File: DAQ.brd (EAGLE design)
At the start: 85.9 x 42.9 mm, 28 parts, among them IC1 PIC18F4550_40, IC2 7805T, Q1 20MHz, X1 PN61729-S

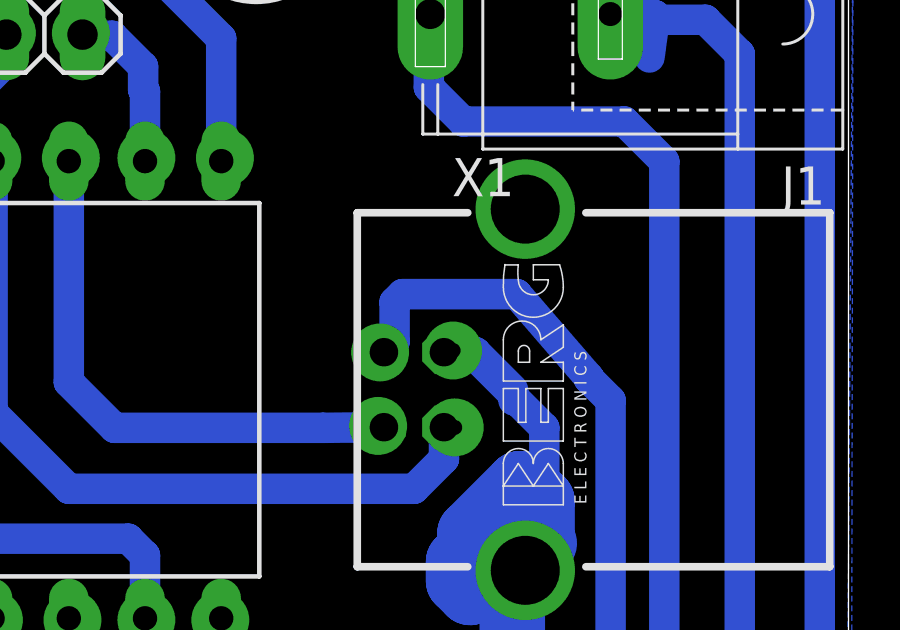
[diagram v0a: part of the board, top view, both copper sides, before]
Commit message: files word
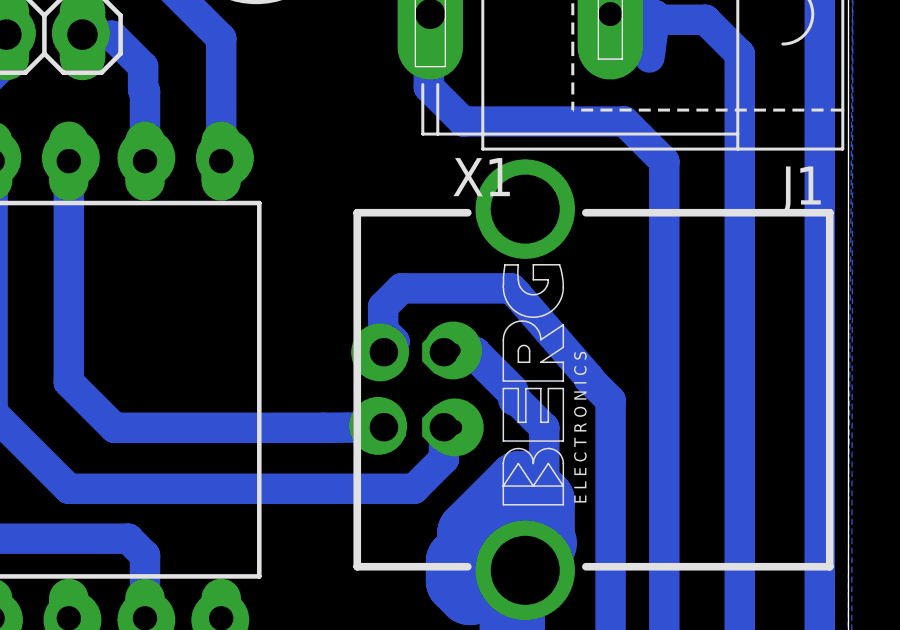
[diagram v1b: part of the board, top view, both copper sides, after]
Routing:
- net +5USB: track 175.3 -> 175.9 mm
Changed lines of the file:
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@@
 <layer number="14" name="Route14" color="1" fill="6" visible="no" active="no"/>
 <layer number="15" name="Route15" color="4" fill="6" visible="no" active="yes"/>
-<layer number="16" name="Bottom" color="1" fill="1" visible="no" active="yes"/>
-<layer number="17" name="Pads" color="2" fill="1" visible="no" active="yes"/>
-<layer number="18" name="Vias" color="2" fill="1" visible="no" active="yes"/>
-<layer number="19" name="Unrouted" color="6" fill="1" visible="no" active="yes"/>
+<layer number="16" name="Bottom" color="1" fill="1" visible="yes" active="yes"/>
+<layer number="17" name="Pads" color="2" fill="1" visible="yes" active="yes"/>
+<layer number="18" name="Vias" color="2" fill="1" visible="yes" active="yes"/>
+<layer number="19" name="Unrouted" color="6" fill="1" visible="yes" active="yes"/>
 <layer number="20" name="Dimension" color="15" fill="1" visible="yes" active="yes"/>
-<layer number="21" name="tPlace" color="7" fill="1" visible="yes" active="yes"/>
-<layer number="22" name="bPlace" color="7" fill="1" visible="yes" active="yes"/>
-<layer number="23" name="tOrigins" color="15" fill="1" visible="yes" active="yes"/>
-<layer number="24" name="bOrigins" color="15" fill="1" visible="yes" active="yes"/>
-<layer number="25" name="tNames" color="7" fill="1" visible="yes" active="yes"/>
-<layer number="26" name="bNames" color="7" fill="1" visible="yes" active="yes"/>
-<layer number="27" name="tValues" color="7" fill="1" visible="yes" active="yes"/>
-<layer number="28" name="bValues" color="7" fill="1" visible="yes" active="yes"/>
+<layer number="21" name="tPlace" color="7" fill="1" visible="no" active="yes"/>
+<layer number="22" name="bPlace" color="7" fill="1" visible="no" active="yes"/>
+<layer number="23" name="tOrigins" color="15" fill="1" visible="no" active="yes"/>
+<layer number="24" name="bOrigins" color="15" fill="1" visible="no" active="yes"/>
+<layer number="25" name="tNames" color="7" fill="1" visible="no" active="yes"/>
+<layer number="26" name="bNames" color="7" fill="1" visible="no" active="yes"/>
+<layer number="27" name="tValues" color="7" fill="1" visible="no" active="yes"/>
+<layer number="28" name="bValues" color="7" fill="1" visible="no" active="yes"/>
 <layer number="29" name="tStop" color="7" fill="3" visible="no" active="yes"/>
 <layer number="30" name="bStop" color="7" fill="6" visible="no" active="yes"/>
@@
 <layer number="48" name="Document" color="7" fill="1" visible="no" active="yes"/>
 <layer number="49" name="Reference" color="7" fill="1" visible="no" active="yes"/>
-<layer number="51" name="tDocu" color="7" fill="1" visible="yes" active="yes"/>
-<layer number="52" name="bDocu" color="7" fill="1" visible="yes" active="yes"/>
+<layer number="51" name="tDocu" color="7" fill="1" visible="no" active="yes"/>
+<layer number="52" name="bDocu" color="7" fill="1" visible="no" active="yes"/>
 <layer number="90" name="Modules" color="5" fill="1" visible="no" active="no"/>
 <layer number="91" name="Nets" color="2" fill="1" visible="no" active="no"/>
@@
 <text x="-24.384" y="45.7581" size="2.1844" layer="16" font="vector" ratio="18" rot="MR0">DAQ USB-HID</text>
 <text x="-8.2296" y="79.8195" size="1.4224" layer="25" font="vector" ratio="16">Rx|Tx</text>
-<dimension x1="-62.1602" y1="86.5315" x2="-61.2648" y2="43.3959" x3="-67.045784375" y3="64.852990625" textsize="1.778" layer="20"/>
 <dimension x1="-63.3476" y1="87.0204" x2="23.1013" y2="86.7156" x3="-20.11785625" y3="88.369253125" textsize="1.778" layer="20"/>
+<dimension x1="-63.3476" y1="87.0204" x2="-63.4746" y2="42.672" x3="-71.564434375" y3="64.869546875" textsize="0.0254" layer="20" visible="yes"/>
 </plain>
 <attributes>
@@
 <wire x1="11.6967" y1="44.4246" x2="12.6873" y2="45.5676" width="1.016" layer="16"/>
 <wire x1="14.2875" y1="66.4464" x2="11.8872" y2="69.2277" width="1.016" layer="16"/>
-<wire x1="11.8872" y1="69.2277" x2="8.0772" y2="69.2277" width="1.016" layer="16"/>
-<wire x1="8.0772" y1="69.2277" x2="7.8105" y2="68.961" width="1.016" layer="16"/>
-<wire x1="7.8105" y1="68.961" x2="7.8105" y2="67.6439" width="1.016" layer="16"/>
 <wire x1="7.8105" y1="67.6439" x2="7.4566" y2="67.29" width="1.016" layer="16"/>
 <wire x1="14.2875" y1="66.4464" x2="14.2875" y2="66.4083" width="1.016" layer="16"/>
@@
 <wire x1="12.8016" y1="54.3306" x2="12.8016" y2="45.6819" width="1.016" layer="16"/>
 <wire x1="12.8016" y1="45.6819" x2="12.6873" y2="45.5676" width="1.016" layer="16"/>
+<wire x1="7.8105" y1="67.6439" x2="7.4295" y2="68.0249" width="1.016" layer="16"/>
+<wire x1="7.4295" y1="68.0249" x2="7.4295" y2="68.8086" width="1.016" layer="16"/>
+<wire x1="11.8872" y1="69.2277" x2="11.6967" y2="69.4182" width="1.016" layer="16"/>
+<wire x1="11.6967" y1="69.4182" x2="8.0391" y2="69.4182" width="1.016" layer="16"/>
+<wire x1="8.0391" y1="69.4182" x2="7.4295" y2="68.8086" width="1.016" layer="16"/>
 </signal>
 <signal name="N$133">
 <via x="3.048" y="80.4291" extent="1-16" drill="0.6" diameter="1.778" shape="octagon"/>
 <via x="-10.4775" y="77.8002" extent="1-16" drill="0.6" diameter="1.778" shape="octagon"/>
+<wire x1="-10.4775" y1="77.8002" x2="3.048" y2="80.4291" width="0" layer="19" extent="1-1"/>
 </signal>
 <signal name="N$134">
